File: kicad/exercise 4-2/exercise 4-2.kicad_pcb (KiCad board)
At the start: 2 copper layers, 40.6 x 24.1 mm, 10 parts, among them J1 Conn_01x02_Male, U1 NE555D

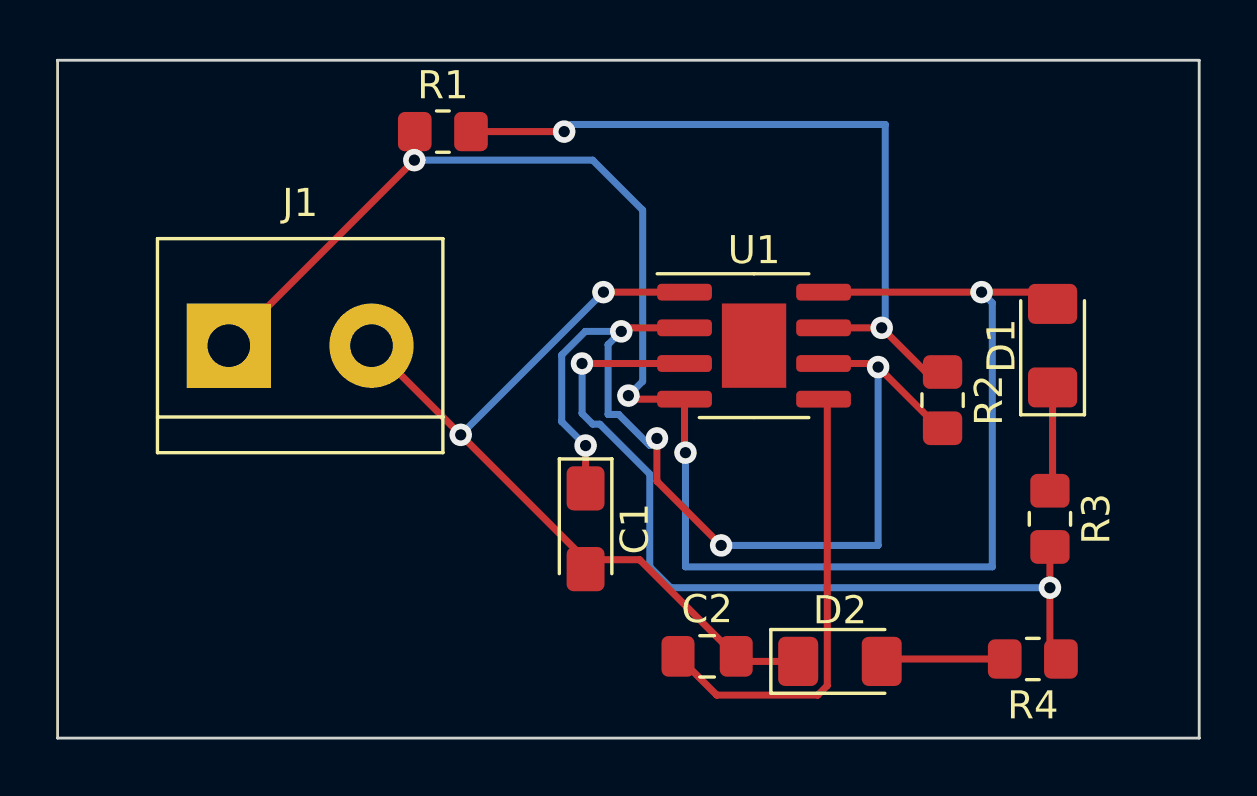
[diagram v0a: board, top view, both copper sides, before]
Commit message: a
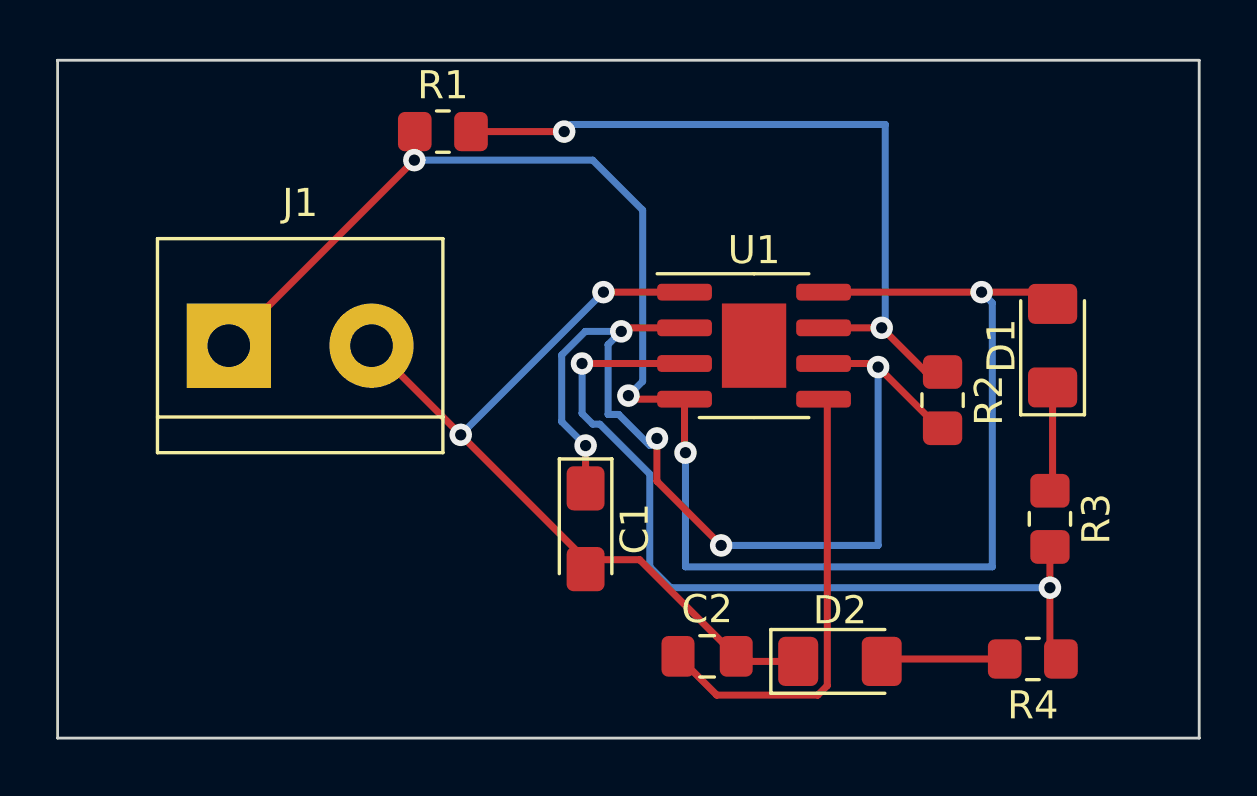
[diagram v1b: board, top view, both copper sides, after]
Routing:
- added copper zone on F.Cu, net (none)
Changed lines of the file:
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@@
       (outputformat 1)
       (mirror false)
-      (drillshape 1)
+      (drillshape 0)
       (scaleselection 1)
       (outputdirectory "")
@@
     (fp_line (start -1 0.625) (end -1 -0.625) (layer "F.Fab") (width 0.1))
     (fp_line (start -1 -0.625) (end 1 -0.625) (layer "F.Fab") (width 0.1))
-    (pad "1" smd roundrect (at -1.0375 0) (size 1.175 1.45) (layers "F.Cu" "F.Paste" "F.Mask") (roundrect_rratio 0.212766)
+    (pad "1" smd roundrect (at -1.0375 0) (size 1.175 1.45) (layers "F.Cu" "F.Paste" "F.Mask") (roundrect_rratio 0.2127659574)
       (net 3 "Net-(C2-Pad1)") (pintype "passive"))
-    (pad "2" smd roundrect (at 1.0375 0) (size 1.175 1.45) (layers "F.Cu" "F.Paste" "F.Mask") (roundrect_rratio 0.212766)
+    (pad "2" smd roundrect (at 1.0375 0) (size 1.175 1.45) (layers "F.Cu" "F.Paste" "F.Mask") (roundrect_rratio 0.2127659574)
       (net 2 "GND") (pintype "passive"))
     (model "${KICAD6_3DMODEL_DIR}/Capacitor_SMD.3dshapes/C_0805_2012Metric.wrl"
@@
     (fp_line (start 1 0.625) (end -1 0.625) (layer "F.Fab") (width 0.1))
     (fp_line (start -1 -0.625) (end 1 -0.625) (layer "F.Fab") (width 0.1))
-    (pad "1" smd roundrect (at -1 0 180) (size 1.2 1.4) (layers "F.Cu" "F.Paste" "F.Mask") (roundrect_rratio 0.208333)
+    (pad "1" smd roundrect (at -1 0 180) (size 1.2 1.4) (layers "F.Cu" "F.Paste" "F.Mask") (roundrect_rratio 0.2083333333)
       (net 8 "/pin_3") (pintype "passive"))
-    (pad "2" smd roundrect (at 1 0 180) (size 1.2 1.4) (layers "F.Cu" "F.Paste" "F.Mask") (roundrect_rratio 0.208333)
+    (pad "2" smd roundrect (at 1 0 180) (size 1.2 1.4) (layers "F.Cu" "F.Paste" "F.Mask") (roundrect_rratio 0.2083333333)
       (net 6 "Net-(D2-Pad2)") (pintype "passive"))
     (model "${KICAD6_3DMODEL_DIR}/Resistor_SMD.3dshapes/R_0805_2012Metric.wrl"
@@
     (fp_line (start 1 -0.625) (end 1 0.625) (layer "F.Fab") (width 0.1))
     (fp_line (start -1 0.625) (end -1 -0.625) (layer "F.Fab") (width 0.1))
-    (pad "1" smd roundrect (at -1 0) (size 1.2 1.4) (layers "F.Cu" "F.Paste" "F.Mask") (roundrect_rratio 0.208333)
+    (pad "1" smd roundrect (at -1 0) (size 1.2 1.4) (layers "F.Cu" "F.Paste" "F.Mask") (roundrect_rratio 0.2083333333)
       (net 5 "+9V") (pintype "passive"))
-    (pad "2" smd roundrect (at 1 0) (size 1.2 1.4) (layers "F.Cu" "F.Paste" "F.Mask") (roundrect_rratio 0.208333)
+    (pad "2" smd roundrect (at 1 0) (size 1.2 1.4) (layers "F.Cu" "F.Paste" "F.Mask") (roundrect_rratio 0.2083333333)
       (net 7 "/pin_7") (pintype "passive"))
     (model "${KICAD6_3DMODEL_DIR}/Resistor_SMD.3dshapes/R_0805_2012Metric.wrl"
@@
     (fp_line (start -1.2 -0.8) (end -1.6 -0.4) (layer "F.Fab") (width 0.1))
     (fp_line (start -1.6 -0.4) (end -1.6 0.8) (layer "F.Fab") (width 0.1))
-    (pad "1" smd roundrect (at -1.4375 0 270) (size 1.575 1.35) (layers "F.Cu" "F.Paste" "F.Mask") (roundrect_rratio 0.185185)
+    (pad "1" smd roundrect (at -1.4375 0 270) (size 1.575 1.35) (layers "F.Cu" "F.Paste" "F.Mask") (roundrect_rratio 0.1851851852)
       (net 1 "/pin_2") (pintype "passive"))
-    (pad "2" smd roundrect (at 1.4375 0 270) (size 1.575 1.35) (layers "F.Cu" "F.Paste" "F.Mask") (roundrect_rratio 0.185185)
+    (pad "2" smd roundrect (at 1.4375 0 270) (size 1.575 1.35) (layers "F.Cu" "F.Paste" "F.Mask") (roundrect_rratio 0.1851851852)
       (net 2 "GND") (pintype "passive"))
     (model "${KICAD6_3DMODEL_DIR}/Capacitor_Tantalum_SMD.3dshapes/CP_EIA-3216-18_Kemet-A.wrl"
@@
     (fp_line (start -1.6 0.8) (end 1.6 0.8) (layer "F.Fab") (width 0.1))
     (fp_line (start 1.6 0.8) (end 1.6 -0.8) (layer "F.Fab") (width 0.1))
-    (pad "1" smd roundrect (at -1.4875 0) (size 1.425 1.75) (layers "F.Cu" "F.Paste" "F.Mask") (roundrect_rratio 0.175439)
+    (pad "1" smd roundrect (at -1.4875 0) (size 1.425 1.75) (layers "F.Cu" "F.Paste" "F.Mask") (roundrect_rratio 0.1754392982)
       (net 2 "GND") (pinfunction "K") (pintype "passive"))
-    (pad "2" smd roundrect (at 1.4875 0) (size 1.425 1.75) (layers "F.Cu" "F.Paste" "F.Mask") (roundrect_rratio 0.175439)
+    (pad "2" smd roundrect (at 1.4875 0) (size 1.425 1.75) (layers "F.Cu" "F.Paste" "F.Mask") (roundrect_rratio 0.1754392982)
       (net 6 "Net-(D2-Pad2)") (pinfunction "A") (pintype "passive"))
     (model "${KICAD6_3DMODEL_DIR}/LED_SMD.3dshapes/LED_1206_3216Metric.wrl"
@@
     (fp_line (start -1 0.625) (end -1 -0.625) (layer "F.Fab") (width 0.1))
     (fp_line (start -1 -0.625) (end 1 -0.625) (layer "F.Fab") (width 0.1))
-    (pad "1" smd roundrect (at -1 0 270) (size 1.2 1.4) (layers "F.Cu" "F.Paste" "F.Mask") (roundrect_rratio 0.208333)
+    (pad "1" smd roundrect (at -1 0 270) (size 1.2 1.4) (layers "F.Cu" "F.Paste" "F.Mask") (roundrect_rratio 0.2083333333)
       (net 7 "/pin_7") (pintype "passive"))
-    (pad "2" smd roundrect (at 1 0 270) (size 1.2 1.4) (layers "F.Cu" "F.Paste" "F.Mask") (roundrect_rratio 0.208333)
+    (pad "2" smd roundrect (at 1 0 270) (size 1.2 1.4) (layers "F.Cu" "F.Paste" "F.Mask") (roundrect_rratio 0.2083333333)
       (net 1 "/pin_2") (pintype "passive"))
     (model "${KICAD6_3DMODEL_DIR}/Resistor_SMD.3dshapes/R_0805_2012Metric.wrl"
@@
     (fp_line (start -1.2 -0.8) (end -1.6 -0.4) (layer "F.Fab") (width 0.1))
     (fp_line (start 1.6 -0.8) (end -1.2 -0.8) (layer "F.Fab") (width 0.1))
-    (pad "1" smd roundrect (at -1.4875 0 90) (size 1.425 1.75) (layers "F.Cu" "F.Paste" "F.Mask") (roundrect_rratio 0.175439)
+    (pad "1" smd roundrect (at -1.4875 0 90) (size 1.425 1.75) (layers "F.Cu" "F.Paste" "F.Mask") (roundrect_rratio 0.1754392982)
       (net 4 "Net-(D1-Pad1)") (pinfunction "K") (pintype "passive"))
-    (pad "2" smd roundrect (at 1.4875 0 90) (size 1.425 1.75) (layers "F.Cu" "F.Paste" "F.Mask") (roundrect_rratio 0.175439)
+    (pad "2" smd roundrect (at 1.4875 0 90) (size 1.425 1.75) (layers "F.Cu" "F.Paste" "F.Mask") (roundrect_rratio 0.1754392982)
       (net 5 "+9V") (pinfunction "A") (pintype "passive"))
     (model "${KICAD6_3DMODEL_DIR}/LED_SMD.3dshapes/LED_1206_3216Metric.wrl"
@@
     (fp_line (start -1 0.625) (end -1 -0.625) (layer "F.Fab") (width 0.1))
     (fp_line (start -1 -0.625) (end 1 -0.625) (layer "F.Fab") (width 0.1))
-    (pad "1" smd roundrect (at -1 0 270) (size 1.2 1.4) (layers "F.Cu" "F.Paste" "F.Mask") (roundrect_rratio 0.208333)
+    (pad "1" smd roundrect (at -1 0 270) (size 1.2 1.4) (layers "F.Cu" "F.Paste" "F.Mask") (roundrect_rratio 0.2083333333)
       (net 4 "Net-(D1-Pad1)") (pintype "passive"))
-    (pad "2" smd roundrect (at 1 0 270) (size 1.2 1.4) (layers "F.Cu" "F.Paste" "F.Mask") (roundrect_rratio 0.208333)
+    (pad "2" smd roundrect (at 1 0 270) (size 1.2 1.4) (layers "F.Cu" "F.Paste" "F.Mask") (roundrect_rratio 0.2083333333)
       (net 8 "/pin_3") (pintype "passive"))
     (model "${KICAD6_3DMODEL_DIR}/Resistor_SMD.3dshapes/R_0805_2012Metric.wrl"
@@
   (segment (start 137.668 73.914) (end 137.414 73.914) (width 0.25) (layer "B.Cu") (net 8))
   (segment (start 140.188 79.736) (end 139.446 78.994) (width 0.25) (layer "B.Cu") (net 8))
+  (zone (net 0) (net_name "") (layer "F.Cu") (hatch edge 0.508)
+    (connect_pads (clearance 0.508))
+    (min_thickness 0.254) (filled_areas_thickness no)
+    (fill yes (thermal_gap 0.508) (thermal_bridge_width 0.508))
+    (polygon
+      (pts
+        (xy 159.004 85.09)
+        (xy 118.364 85.09)
+        (xy 118.364 60.96)
+        (xy 159.004 60.96)
+      )
+    )
+  )
 )
